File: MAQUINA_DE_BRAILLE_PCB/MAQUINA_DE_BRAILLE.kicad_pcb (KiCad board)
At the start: 4 copper layers, 84.5 x 81.1 mm, 73 parts, among them J1 Screw_Terminal_01x04, J2 Screw_Terminal_01x04, J3 Screw_Terminal_01x02, J4 USB_C_Receptacle_USB2.0_16P, J5 Screw_Terminal_01x03, J6 Screw_Terminal_01x03, J7 Screw_Terminal_01x02, J8 Screw_Terminal_01x16, Q1 IRLZ44NSTRLPBF, U1 ESP32-S3-WROOM-1-N16, U2 DRV8825PWPR, U3 DRV8825PWPR

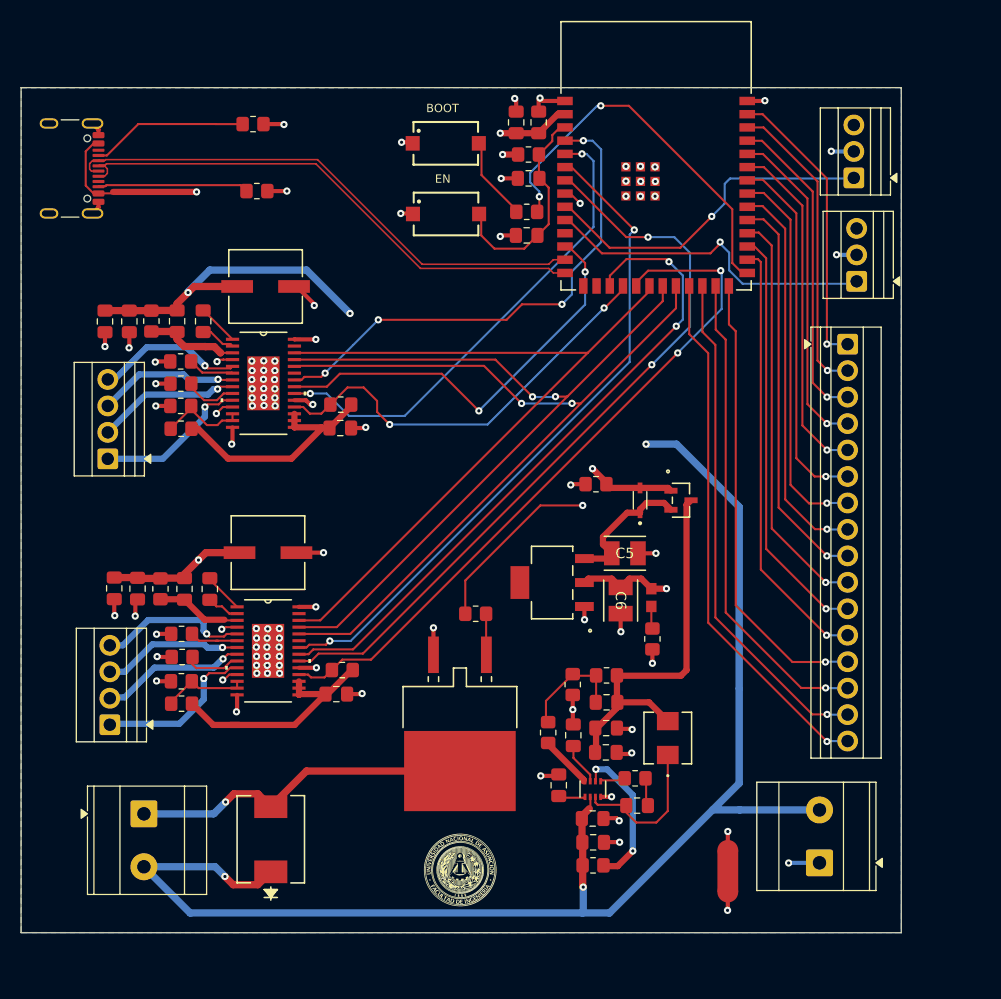
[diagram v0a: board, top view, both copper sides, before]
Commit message: a
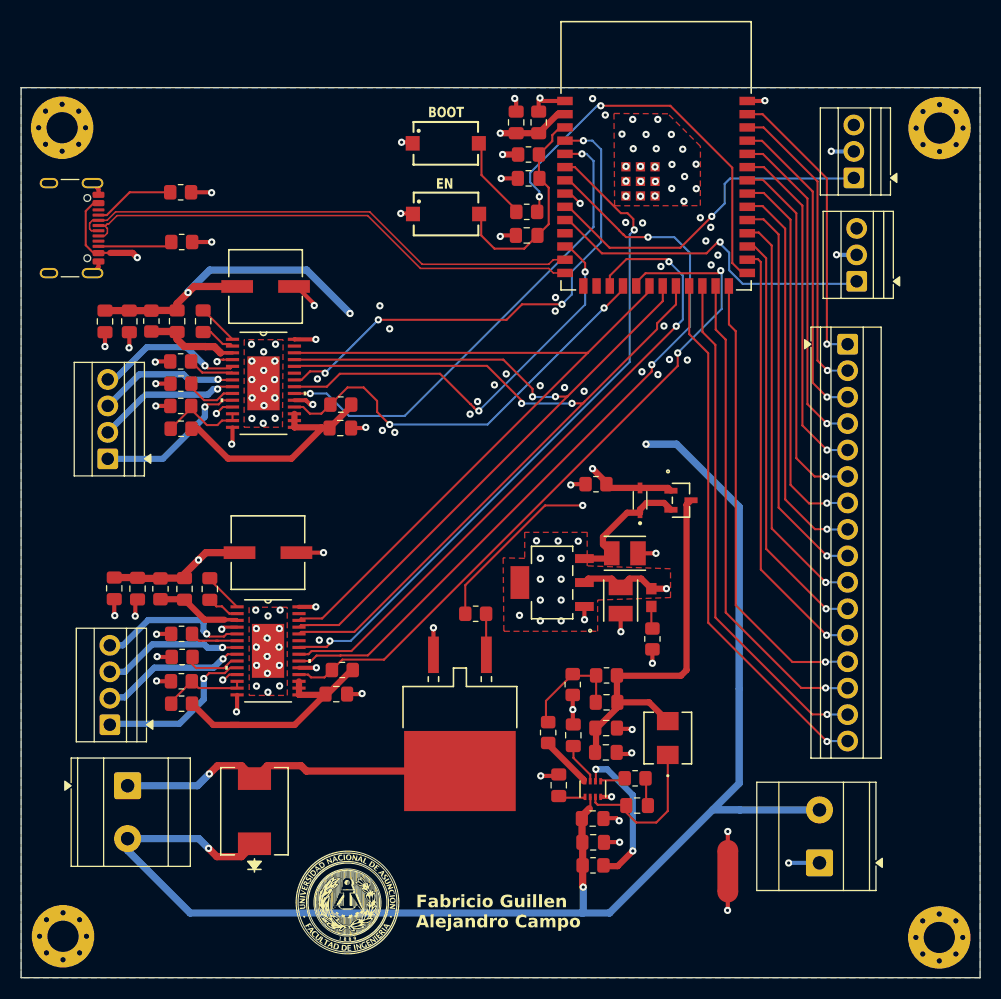
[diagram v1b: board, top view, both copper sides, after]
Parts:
- added H1: MountingHole_Pad, MountingHole:MountingHole_3mm_Pad_Via, F.Cu at (110.6, 48.2)
- added H2: MountingHole_Pad, MountingHole:MountingHole_3mm_Pad_Via, F.Cu at (194.8, 48.2)
- added H3: MountingHole_Pad, MountingHole:MountingHole_3mm_Pad_Via, F.Cu at (110.7, 125.8)
- added H4: MountingHole_Pad, MountingHole:MountingHole_3mm_Pad_Via, F.Cu at (194.8, 125.9)
- moved G*** 11.3 mm to (138.0, 122.6)
- moved R2 9.55 mm to (122.0, 54.4)
- moved R3 8.72 mm to (122.1, 59.1)
- moved J4 5.73 mm to (110.4, 57.8)
- moved J7 3.12 mm to (116.9, 111.3)
- moved CR1 3.12 mm to (129.1, 113.8)
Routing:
- net Net-(J4-CC2): track 14.5 -> 7.16 mm
- net Net-(J4-CC1): track 15.2 -> 7.85 mm
- net USB_TO_MOSFET: track 73.6 -> 70.2 mm
- net VCC: track 274.5 -> 277.9 mm
- net USB_D+: track 51.6 -> 48.7 mm
- net BOOT: track 37.4 -> 39.7 mm
- net USB_D-: track 51.8 -> 49.8 mm
- net GNDD: track 25.4 -> 26.2 mm, vias 21 -> 65
- net Net-(J7-Pin_1): track 33.1 -> 33.9 mm
- net DRIVER_Y_nFAULT_TO_ESP32: track 68.6 -> 69.3 mm
- net DRIVER_Y_STEP_TO_ESP32: track 65.1 -> 65.8 mm
- net MODE0_TO_ESP32: track 79.6 -> 80.3 mm
- net VCC_3V3: vias 3 -> 15
- net GND: vias 71 -> 65
- added copper zone on F.Cu, net GND
- added copper zone on F.Cu, net GNDD
- added copper zone on F.Cu, net VCC_3V3
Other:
- board size 84.5 x 81.1 mm -> 92.1 x 85.4 mm
- board text added: "Fabricio Guillen Alejandro Campo"
